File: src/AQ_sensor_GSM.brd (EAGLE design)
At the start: 110 x 64 mm, 120 parts, among them IC1 MIC29302WU, J1 F-1X03-SIP-100-32, J3 PJ-002BH, Q1 MMBT2222, Q2 MMBT2222, Q3 MMBT2222, Q4 MMBT2222, Q5 MMBT2222, Q6 MMBT2222, Q7 MMBT2222, U3 TEXAS_INSTRUMENTS_LM1117IMP-3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, U5 TXS0108EPWR, X1 53048-08

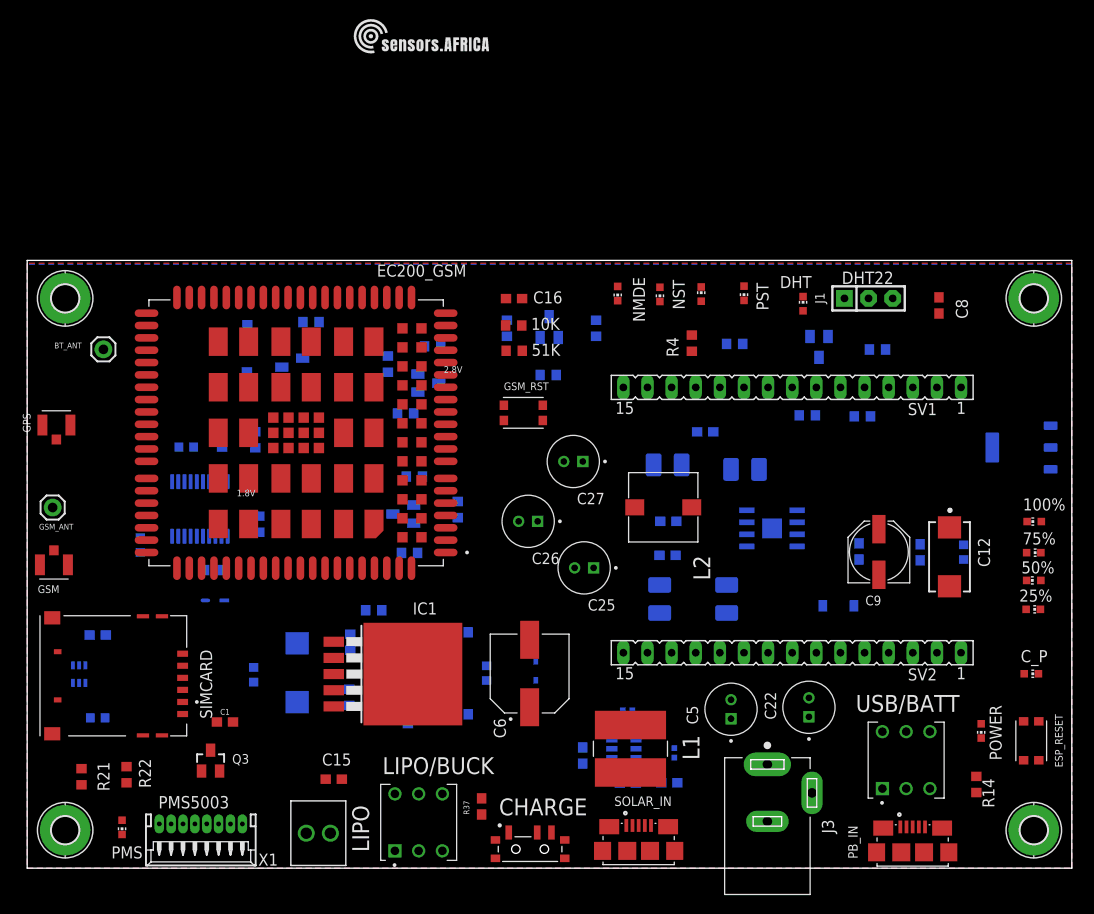
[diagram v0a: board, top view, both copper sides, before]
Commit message: Routed
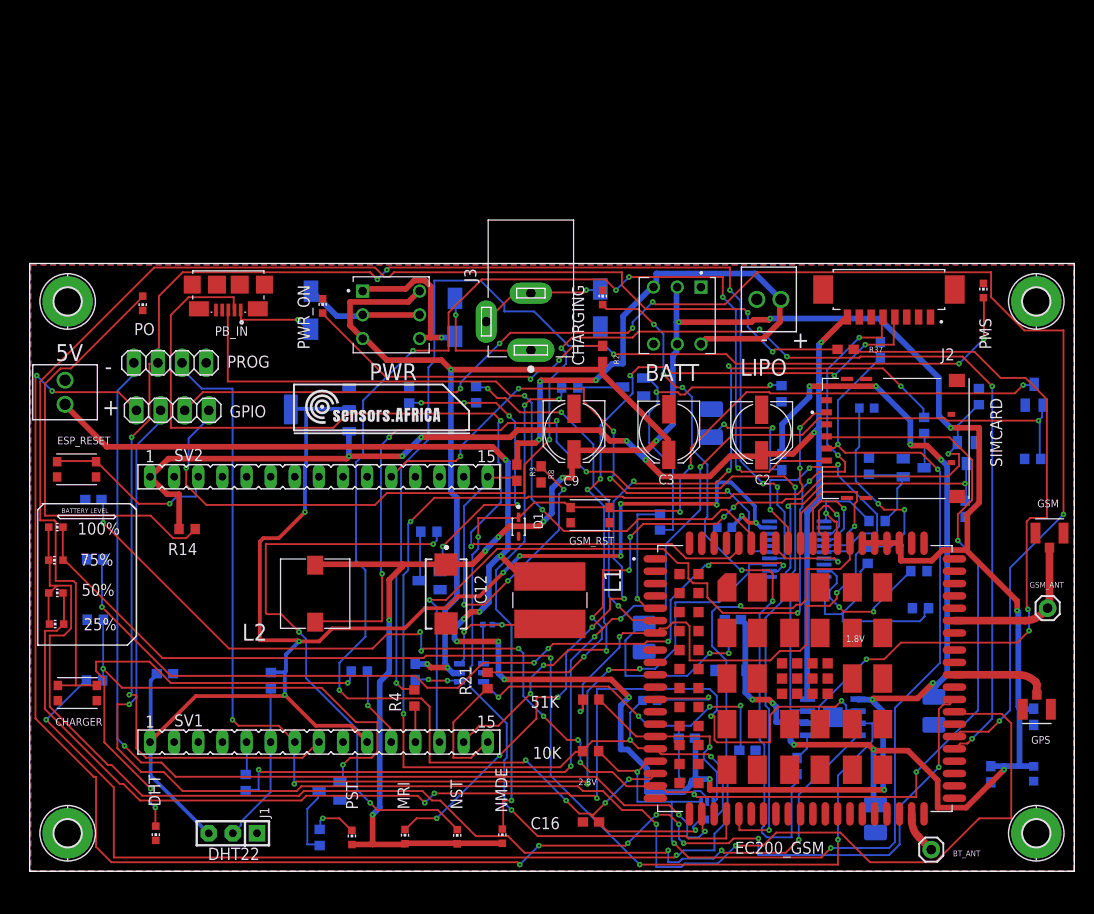
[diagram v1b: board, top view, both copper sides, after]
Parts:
- removed C22, C25, C26, C27, C5: ECA-1HM220, Resistor_Capacitor:CAP_RADIAL_2MM
- removed C6: EEEFN1C471P, EEEFN1C471P:CAP_EEEFN1C471P
- removed C7: 100nf, 06035C104K4T2A:CAPC1608X90N
- removed CHARGE: PCM12SMTR, AQ_sensor_MRC:SW_PCM12SMTR
- removed C_P: ORANGE, led:CHIP-LED0603
- removed D5: ESD56151W04, 4.7V TVS Diode:DIO_1N4148WS_RR
- removed IC1: MIC29302WU, MIC29302WU:TO263-5
- removed LIPO/BUCK, USB/BATT: TL2285EE, TL2285EE:SW_TL2285EE
- removed POWER: RED, led:CHIP-LED0603
- removed Q1: MMBT2222, MMBT2222_:SOT23-BEC
- removed R10: 47K, rcl:R0603
- removed R11: 470R, rcl:R0603
- removed R9: 100k, rcl:R0603
- removed SOLAR_IN: 10118192-0001LF, AQ_sensor_GSM:AMPHENOL_10118192-0001LF
- removed U$1: (no value), MT2492:SOT95P280X145-6N
- removed X1: 53048-08, AQ_sensor_GSM:53048-08
- added 5V: 2828XX-2282834-2, Connector:TERMBLK_254-2N
- added BATT, PWR: TL2285EE, TL2285EE:SW_TL2285EE
- added CHARGER: KMR621NGLFS, AQ_sensor_GSM:SW_KMR621NGLFS
- added CHARGING, PWR_ON: ORANGE, led:CHIP-LED0603
- added D4, D6, D7: SS54-HF, SS54-HF schottkey Diode:DIOM5025X220N
- added GPIO, PROG: PINHD-1X4, Connector:1X04
- added J2: 53261-0871, 53261-0871:MOLEX_53261-0871
- added MT2492: MT2492, MT2492:SOT95P280X145-6N
- added PO: RED, led:CHIP-LED0603
- C2: value 470uf -> 100uF; device T495X477K010ATE100:CAPMP7343X430N -> rcl:PANASONIC_D
- C3: value 100nf -> 100uF; device 06035C104K4T2A:CAPC1608X90N -> rcl:PANASONIC_D
- R2: value 51K -> 1k; device rcl:R0603 -> SparkFun-Resistors:0603
- R3: value 4.7K -> 47k; device rcl:R0603 -> SparkFun-Resistors:0603
- R8: value 47K -> 10k; device rcl:R0603 -> SparkFun-Resistors:0603
- moved H3 116.7 mm to (106.3, 3.68), turned to 180 degrees
- moved H4 116.4 mm to (106.3, 59.7), turned to 180 degrees
- moved H2 116.3 mm to (4.26, 3.68), turned to 180 degrees
- moved H1 116.0 mm to (4.26, 59.7), turned to 180 degrees
- moved GPS 107.5 mm to (106.3, 16.7), turned to 180 degrees
- moved PMS 106.9 mm to (100.7, 60.8), turned to 0 degrees
- moved GSM_ANT 105.3 mm to (107.5, 27.4), turned to 180 degrees
- moved GSM 104.9 mm to (107.7, 35.3), turned to 0 degrees
- moved ESP_RESET 104.5 mm to (5.21, 42.0), turned to 180 degrees
- moved 100% 103.0 mm to (3.02, 35.9), turned to 270 degrees
- moved 50% 103.0 mm to (3.02, 29.0), turned to 270 degrees
- moved 75% 103.0 mm to (3.02, 32.4), turned to 90 degrees
- moved 25% 102.9 mm to (3.10, 25.7), turned to 90 degrees
- moved BT_ANT 101.9 mm to (95.2, 1.96), turned to 180 degrees
- moved R22 98.2 mm to (100.2, 49.7), flipped to the bottom
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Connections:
- net USB_VBUS renamed G_USB_VBUS
- removed net +5V: R14.2, SV2.1, U3.3, USB/BATT.3, USB/BATT.4, X1.8
- removed net 3.8V: C6.1, C7.2, D5.C, IC1.4, LIPO/BUCK.1, LIPO/BUCK.6, R11.2, R9.2
- removed net 4.2V: C29.1, L2.2, LIPO/BUCK.2, LIPO/BUCK.5, R19.2, U$2.6
- removed net BVIN: C5.1, J3.1, R7.2, SOLAR_IN.1, U$1.5
- removed net D+: PB_IN.3, SOLAR_IN.3
- removed net D-: PB_IN.2, SOLAR_IN.2
- removed net N$36: Q1.B, R3.2
- removed net N$37: Q1.E, R8.2
- removed net N$38: IC1.5, R10.2, R9.1
- removed net TF-CLK: SV2.7
- removed net TF-CS: SV2.9
- removed net TF-MISO: SV2.8
- removed net TF-MOSI: SV2.10
- new net 4.5-16V: C3.+, MT2492.5, PWR.3, PWR.4, R2.1, R7.2
- new net 5VT: D4.1, PWR.2, PWR.5
- new net BMSV: R3.2, R8.1, SV2.15
- new net G_ADC0: EC200_GSM.45, GPIO.1
- new net G_ADC1: EC200_GSM.44, GPIO.2
- new net G_ADC2: EC200_GSM.43
- new net G_GPIO1: EC200_GSM.126
- new net G_I2C_SCL: EC200_GSM.41, GPIO.4
- new net G_I2C_SDA: EC200_GSM.42, GPIO.3
- new net G_SPI_CLK: EC200_GSM.40
- new net G_SPI_CS: EC200_GSM.37
- new net G_SPI_MISO: EC200_GSM.39
- new net G_SPI_MOSI: EC200_GSM.38
- new net G_USB_BOOT: EC200_GSM.115, PROG.1
- new net G_USB_D+: EC200_GSM.69, PB_IN.3
- new net G_USB_D-: EC200_GSM.70, PB_IN.2
- new net LBV: BATT.3, BATT.4, LIPO.1, R3.1
- new net N$59: D4.2, PB_IN.1
- new net N$60: D7.1, J3.2, J3.3
- new net N$61: D6.2, J3.1
- net 5V_IN: now also 5V.1; no longer C22.1
- net 5V_OUT: now also C2.+, J2.8, R14.2, SV2.1, U3.3; no longer C25.1, C26.1, C27.1, USB/BATT.2, USB/BATT.5
- net GND: now also 5V.2, C2.-, C3.-, CHARGER.2_1, CHARGER.2_2, CHARGING.C, D7.2, J2.7, MT2492.2, PO.C, PROG.4, PWR_ON.C, R8.2; no longer C2.2, C22.2, C25.2, C26.2, C27.2, C3.1, C5.2, C6.2, C7.1, CHARGE.2, C_P.C, D5.A, IC1.3, J3.2, J3.3, POWER.C, R10.1, R11.1, R8.1, SOLAR_IN.4, SOLAR_IN.5, SOLAR_IN.SH1, SOLAR_IN.SH2, SOLAR_IN.SH3, SOLAR_IN.SH4, SOLAR_IN.SH5, SOLAR_IN.SH6, U$1.2, X1.7
- net MCU_RXD: now also PROG.2
- net MCU_TXD: now also PROG.3
- net N$10: now also MT2492.3; no longer U$1.3
- net N$11: now also MT2492.4; no longer U$1.4
- net N$20: now also CHARGER.1_1, CHARGER.1_2; no longer CHARGE.1
- net N$25: now also PO.A; no longer POWER.A
- net N$3: now also MT2492.1; no longer U$1.1
- net N$35: now also PWR_ON.A, R2.2; no longer IC1.1, Q1.C, R2.1
- net N$46: now also CHARGING.A; no longer C_P.A
- net N$6: now also MT2492.6; no longer U$1.6
- net PMS_RX: now also J2.5; no longer X1.5
- net PMS_TX: now also J2.4; no longer X1.4
- net VBAT_EN: no longer R3.1
- net VUSB: now also D6.1, PWR.1, PWR.6; no longer C2.1, C3.2, IC1.2, PB_IN.1, R2.2, USB/BATT.1, USB/BATT.6
- net V_LIPO: now also BATT.2, BATT.5, C29.1, L2.2, R19.2, U$2.6; no longer LIPO.1, LIPO/BUCK.3, LIPO/BUCK.4
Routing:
- net V_LIPO: track 0.00 -> 258.7 mm, vias 0 -> 16
- net 5V_IN: track 0.00 -> 214.6 mm, vias 0 -> 16
- net G_ADC0: track 0.00 -> 174.7 mm, vias 0 -> 10
- net MCU_RXD: track 0.00 -> 167.8 mm, vias 0 -> 7
- net SIMCLK: track 0.00 -> 167.2 mm, vias 0 -> 11
- net SIMRST: track 0.00 -> 165.3 mm, vias 0 -> 10
- net G_ADC1: track 0.00 -> 161.7 mm, vias 0 -> 3
- net +3V3: track 0.00 -> 159.7 mm, vias 0 -> 10
- net G_I2C_SDA: track 0.00 -> 152.9 mm, vias 0 -> 6
- net G_I2C_SCL: track 0.00 -> 152.2 mm, vias 0 -> 7
- net N$20: track 0.00 -> 134.4 mm, vias 0 -> 2
- net PWRSTAT: track 0.00 -> 133.9 mm, vias 0 -> 3
- net N$14: track 0.00 -> 129.3 mm, vias 0 -> 3
- net 5V_OUT: track 0.00 -> 128.7 mm, vias 0 -> 7
- net GSM_RST: track 0.00 -> 128.3 mm, vias 0 -> 5
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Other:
- board text added: "+"
- board text added: "-"
- board text added: "BATTERY LEVEL"
- board text removed: "PMS5003"
